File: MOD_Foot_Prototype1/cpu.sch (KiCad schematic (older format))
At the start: 18 parts, among them CN1 CONN_PANNEL_2X2, CN2 CONN_PANNEL_2X2, P1 HEADER_5X2, P2 HEADER_5X2, U2 LPC111X_LQFP48, X1 10MHz

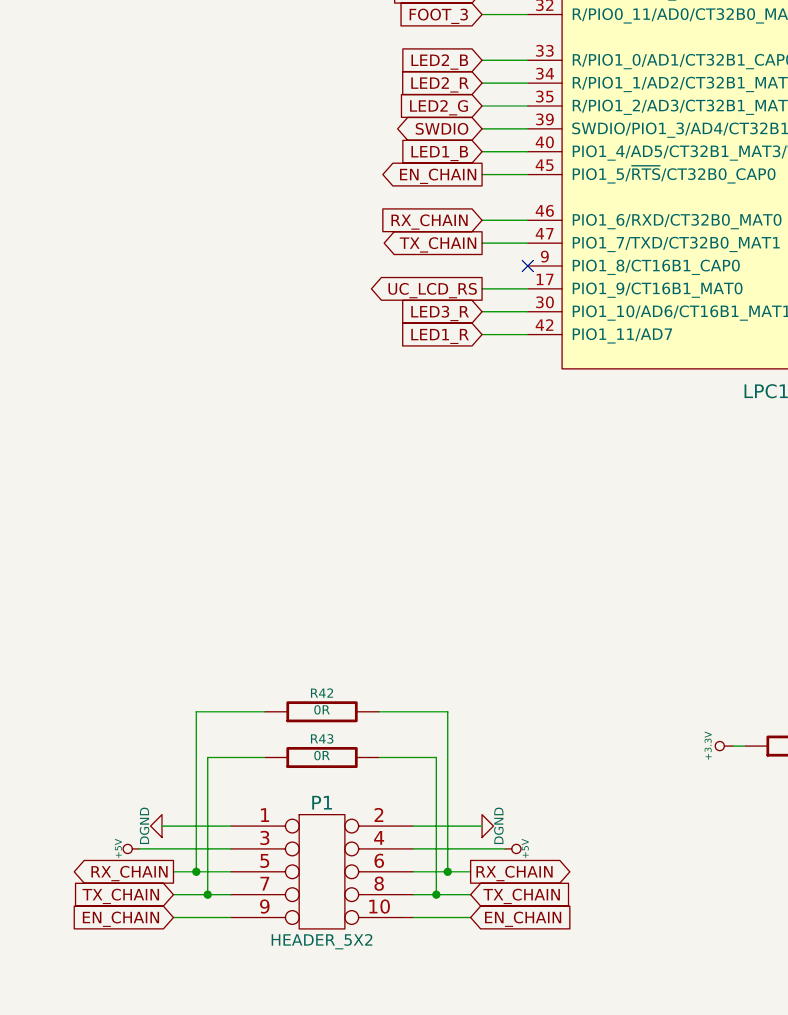
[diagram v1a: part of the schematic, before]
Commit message: yet about issue #11: sch: pins 9 and 10 are being connected with 0R resitor
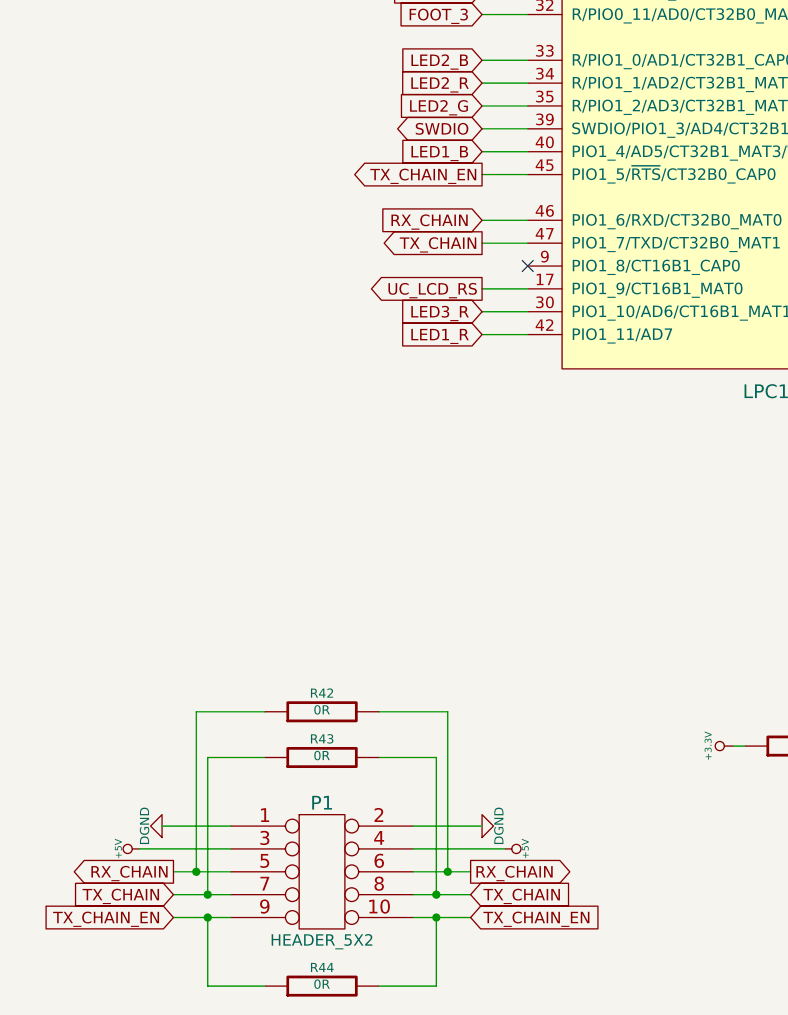
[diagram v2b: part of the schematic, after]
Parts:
- added R44: 0R, MOD_Footprints_Lib:SM0805, symbol R
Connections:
- net EN_CHAIN renamed TX_CHAIN_EN
- net TX_CHAIN_EN: now also R44.1, R44.2
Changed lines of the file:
@@
 RX_CHAIN
 Text GLabel 2650 3450 0    50   Output ~ 0
-EN_CHAIN
+TX_CHAIN_EN
 Text GLabel 2650 3950 0    50   Output ~ 0
 UC_LCD_RS
@@
 $EndComp
 Text GLabel 1300 6700 0    50   Input ~ 0
-EN_CHAIN
+TX_CHAIN_EN
 NoConn ~ 2850 2150
 NoConn ~ 2850 1750
@@
 TX_CHAIN
 Text GLabel 2600 6700 2    50   Input ~ 0
-EN_CHAIN
+TX_CHAIN_EN
 $Comp
 L R R42
@@
 	2500 5800 2500 6500
 Connection ~ 2500 6500
+$Comp
+L R R44
+U 1 1 548854D0
+P 1950 7000
+F 0 "R44" V 2030 7000 40  0000 C CNN
+F 1 "0R" V 1957 7001 40  0000 C CNN
+F 2 "MOD_Footprints_Lib:SM0805" V 1880 7000 30  0001 C CNN
+F 3 "~" H 1950 7000 30  0000 C CNN
+	1    1950 7000
+	0    -1   -1   0
+$EndComp
+Wire Wire Line
+	1700 7000 1450 7000
+Wire Wire Line
+	1450 7000 1450 6700
+Connection ~ 1450 6700
+Wire Wire Line
+	2200 7000 2450 7000
+Wire Wire Line
+	2450 7000 2450 6700
+Connection ~ 2450 6700
 $EndSCHEMATC

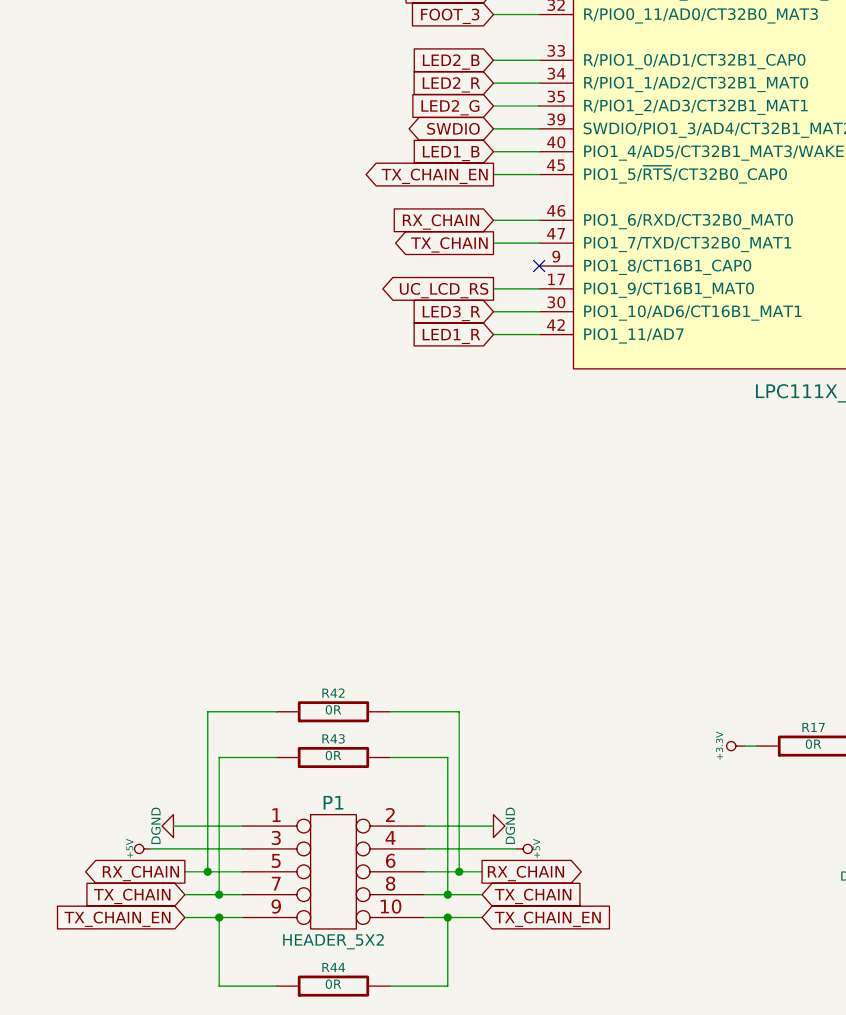
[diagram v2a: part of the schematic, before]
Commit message: * fix wrong control-chain signal names * annotate new resistors added to the sch * rearrange sch drawing around header P1
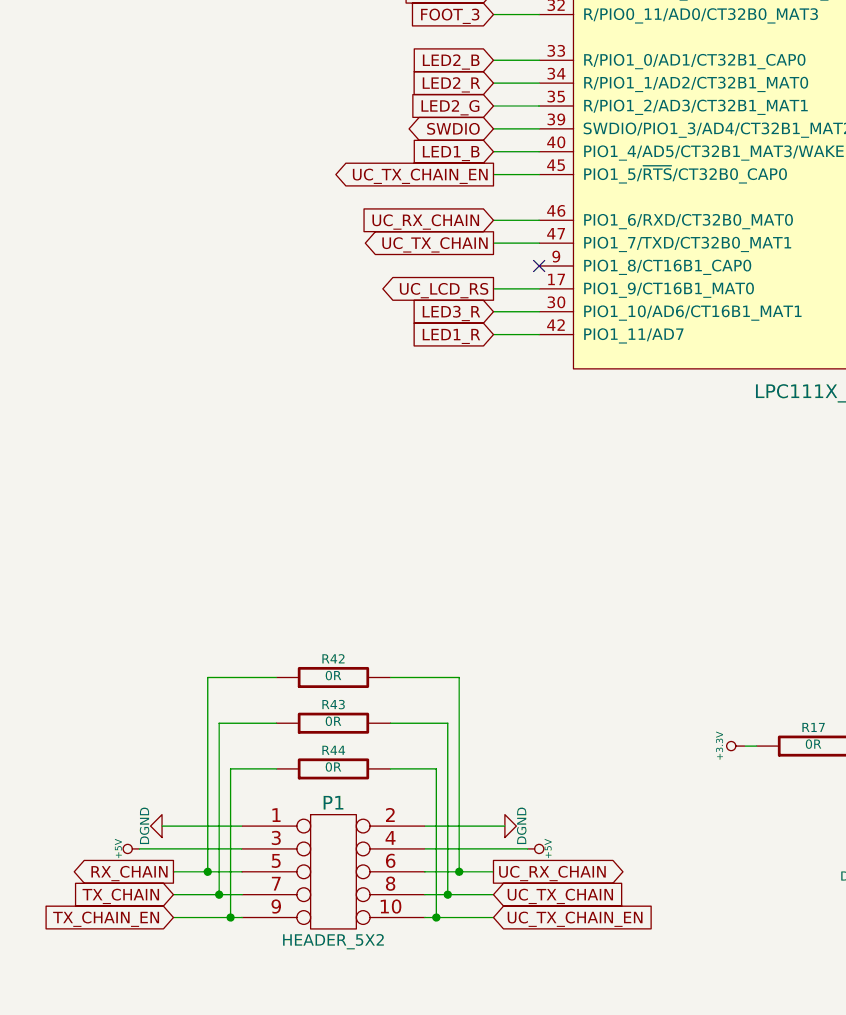
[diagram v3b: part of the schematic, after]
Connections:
- net RX_CHAIN: no longer P1.6, R42.2, U2.46 (PIO1_6/RXD/CT32B0_MAT0)
- net TX_CHAIN: no longer P1.8, R43.2, U2.47 (PIO1_7/TXD/CT32B0_MAT1)
- net TX_CHAIN_EN: no longer P1.10, R44.2, U2.45 (PIO1_5/~RTS~/CT32B0_CAP0)
- new net UC_RX_CHAIN: P1.6, R42.2, U2.46 (PIO1_6/RXD/CT32B0_MAT0)
- new net UC_TX_CHAIN: P1.8, R43.2, U2.47 (PIO1_7/TXD/CT32B0_MAT1)
- new net UC_TX_CHAIN_EN: P1.10, R44.2, U2.45 (PIO1_5/~RTS~/CT32B0_CAP0)
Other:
- moved on the sheet: R42, R43, R44
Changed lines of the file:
@@
 $EndComp
 $Comp
-L DGND #PWR021
+L DGND #PWR30
 U 1 1 54834712
 P 5550 4000
-F 0 "#PWR021" H 5550 4000 40  0001 C CNN
+F 0 "#PWR30" H 5550 4000 40  0001 C CNN
 F 1 "DGND" H 5550 3930 40  0000 C CNN
 F 2 "" H 5550 4000 60  0000 C CNN
@@
 $EndComp
 $Comp
-L DGND #PWR022
+L DGND #PWR35
 U 1 1 5483471F
 P 6550 3600
-F 0 "#PWR022" H 6550 3600 40  0001 C CNN
+F 0 "#PWR35" H 6550 3600 40  0001 C CNN
 F 1 "DGND" H 6550 3530 40  0000 C CNN
 F 2 "" H 6550 3600 60  0000 C CNN
@@
 $EndComp
 $Comp
-L DGND #PWR023
+L DGND #PWR34
 U 1 1 54834725
 P 6550 3400
-F 0 "#PWR023" H 6550 3400 40  0001 C CNN
+F 0 "#PWR34" H 6550 3400 40  0001 C CNN
 F 1 "DGND" H 6550 3330 40  0000 C CNN
 F 2 "" H 6550 3400 60  0000 C CNN
@@
 $EndComp
 $Comp
-L +3.3V #PWR024
+L +3.3V #PWR31
 U 1 1 5483472B
 P 5950 3350
-F 0 "#PWR024" H 5950 3310 30  0001 C CNN
+F 0 "#PWR31" H 5950 3310 30  0001 C CNN
 F 1 "+3.3V" H 5950 3460 30  0000 C CNN
 F 2 "" H 5950 3350 60  0000 C CNN
@@
 $EndComp
 $Comp
-L DGND #PWR025
+L DGND #PWR33
 U 1 1 5483473F
 P 6350 4900
-F 0 "#PWR025" H 6350 4900 40  0001 C CNN
+F 0 "#PWR33" H 6350 4900 40  0001 C CNN
 F 1 "DGND" H 6350 4830 40  0000 C CNN
 F 2 "" H 6350 4900 60  0000 C CNN
@@
 $EndComp
 $Comp
-L DGND #PWR026
+L DGND #PWR32
 U 1 1 54834745
 P 6350 4100
-F 0 "#PWR026" H 6350 4100 40  0001 C CNN
+F 0 "#PWR32" H 6350 4100 40  0001 C CNN
 F 1 "DGND" H 6350 4030 40  0000 C CNN
 F 2 "" H 6350 4100 60  0000 C CNN
@@
 $EndComp
 $Comp
-L DGND #PWR027
+L DGND #PWR24
 U 1 1 54834760
 P 2150 1400
-F 0 "#PWR027" H 2150 1400 40  0001 C CNN
+F 0 "#PWR24" H 2150 1400 40  0001 C CNN
 F 1 "DGND" H 2150 1330 40  0000 C CNN
 F 2 "" H 2150 1400 60  0000 C CNN
@@
 $EndComp
 $Comp
-L +3.3V #PWR028
+L +3.3V #PWR26
 U 1 1 54834766
 P 2750 800
-F 0 "#PWR028" H 2750 760 30  0001 C CNN
+F 0 "#PWR26" H 2750 760 30  0001 C CNN
 F 1 "+3.3V" H 2750 910 30  0000 C CNN
 F 2 "" H 2750 800 60  0000 C CNN
@@
 SWDCLK
 $Comp
-L DGND #PWR029
+L DGND #PWR29
 U 1 1 54834777
 P 4250 6450
-F 0 "#PWR029" H 4250 6450 40  0001 C CNN
+F 0 "#PWR29" H 4250 6450 40  0001 C CNN
 F 1 "DGND" H 4250 6380 40  0000 C CNN
 F 2 "" H 4250 6450 60  0000 C CNN
@@
 NoConn ~ 5150 6250
 Text GLabel 2650 3750 0    50   Output ~ 0
-TX_CHAIN
+UC_TX_CHAIN
 Text GLabel 2650 3650 0    50   Input ~ 0
-RX_CHAIN
+UC_RX_CHAIN
 Text GLabel 2650 3450 0    50   Output ~ 0
-TX_CHAIN_EN
+UC_TX_CHAIN_EN
 Text GLabel 2650 3950 0    50   Output ~ 0
 UC_LCD_RS
@@
 Text GLabel 5650 3100 2    50   Output ~ 0
 LED5
-Text GLabel 1300 6500 0    50   Output ~ 0
+Text GLabel 1250 6500 0    50   Output ~ 0
 RX_CHAIN
-Text GLabel 1300 6600 0    50   Input ~ 0
+Text GLabel 1250 6600 0    50   Input ~ 0
 TX_CHAIN
 $Comp
-L +5V #PWR030
+L +5V #PWR21
 U 1 1 5483479B
-P 1150 6400
-F 0 "#PWR030" H 1150 6490 20  0001 C CNN
-F 1 "+5V" H 1150 6490 30  0000 C CNN
-F 2 "" H 1150 6400 60  0000 C CNN
-F 3 "" H 1150 6400 60  0000 C CNN
-	1    1150 6400
-	0    -1   -1   0
-$EndComp
-$Comp
-L DGND #PWR031
+P 1100 6400
+F 0 "#PWR21" H 1100 6490 20  0001 C CNN
+F 1 "+5V" H 1100 6490 30  0000 C CNN
+F 2 "" H 1100 6400 60  0000 C CNN
+F 3 "" H 1100 6400 60  0000 C CNN
+	1    1100 6400
+	0    -1   -1   0
+$EndComp
+$Comp
+L DGND #PWR22
 U 1 1 548347A1
-P 1250 6300
-F 0 "#PWR031" H 1250 6300 40  0001 C CNN
-F 1 "DGND" H 1250 6225 40  0000 C CNN
-F 2 "" H 1250 6300 60  0000 C CNN
-F 3 "" H 1250 6300 60  0000 C CNN
-	1    1250 6300
+P 1200 6300
+F 0 "#PWR22" H 1200 6300 40  0001 C CNN
+F 1 "DGND" H 1200 6225 40  0000 C CNN
+F 2 "" H 1200 6300 60  0000 C CNN
+F 3 "" H 1200 6300 60  0000 C CNN
+	1    1200 6300
 	0    1    -1   0
 $EndComp
@@
 $EndComp
 $Comp
-L +3.3V #PWR032
+L +3.3V #PWR23
 U 1 1 548347AE
 P 1800 1650
-F 0 "#PWR032" H 1800 1610 30  0001 C CNN
+F 0 "#PWR23" H 1800 1610 30  0001 C CNN
 F 1 "+3.3V" H 1800 1760 30  0000 C CNN
 F 2 "" H 1800 1650 60  0000 C CNN
@@
 $EndComp
 $Comp
-L +3.3V #PWR033
+L +3.3V #PWR28
 U 1 1 54834827
 P 3750 5950
-F 0 "#PWR033" H 3750 5910 30  0001 C CNN
+F 0 "#PWR28" H 3750 5910 30  0001 C CNN
 F 1 "+3.3V" H 3750 6060 30  0000 C CNN
 F 2 "" H 3750 5950 60  0000 C CNN
@@
 	0    -1   -1   0
 $EndComp
-Text GLabel 1300 6700 0    50   Input ~ 0
+Text GLabel 1250 6700 0    50   Input ~ 0
 TX_CHAIN_EN
 NoConn ~ 2850 2150
@@
 NoConn ~ 5450 3300
 $Comp
-L DGND #PWR034
+L DGND #PWR36
 U 1 1 5483484A
 P 7350 5950
-F 0 "#PWR034" H 7350 5950 40  0001 C CNN
+F 0 "#PWR36" H 7350 5950 40  0001 C CNN
 F 1 "DGND" H 7350 5880 40  0000 C CNN
 F 2 "" H 7350 5950 60  0000 C CNN
@@
 $EndComp
 $Comp
-L DGND #PWR035
+L DGND #PWR37
 U 1 1 54834850
 P 8350 5950
-F 0 "#PWR035" H 8350 5950 40  0001 C CNN
+F 0 "#PWR37" H 8350 5950 40  0001 C CNN
 F 1 "DGND" H 8350 5880 40  0000 C CNN
 F 2 "" H 8350 5950 60  0000 C CNN
@@
 $EndComp
 $Comp
-L +5V #PWR036
+L +5V #PWR27
 U 1 1 548788DF
-P 2750 6400
-F 0 "#PWR036" H 2750 6490 20  0001 C CNN
-F 1 "+5V" H 2750 6490 30  0000 C CNN
-F 2 "" H 2750 6400 60  0000 C CNN
-F 3 "" H 2750 6400 60  0000 C CNN
-	1    2750 6400
+P 2800 6400
+F 0 "#PWR27" H 2800 6490 20  0001 C CNN
+F 1 "+5V" H 2800 6490 30  0000 C CNN
+F 2 "" H 2800 6400 60  0000 C CNN
+F 3 "" H 2800 6400 60  0000 C CNN
+	1    2800 6400
 	0    1    -1   0
 $EndComp
 $Comp
-L DGND #PWR037
+L DGND #PWR25
 U 1 1 548788E5
-P 2650 6300
-F 0 "#PWR037" H 2650 6300 40  0001 C CNN
-F 1 "DGND" H 2650 6225 40  0000 C CNN
-F 2 "" H 2650 6300 60  0000 C CNN
-F 3 "" H 2650 6300 60  0000 C CNN
-	1    2650 6300
-	0    -1   -1   0
-$EndComp
-Text GLabel 2600 6500 2    50   Output ~ 0
-RX_CHAIN
-Text GLabel 2600 6600 2    50   Input ~ 0
-TX_CHAIN
-Text GLabel 2600 6700 2    50   Input ~ 0
-TX_CHAIN_EN
+P 2700 6300
+F 0 "#PWR25" H 2700 6300 40  0001 C CNN
+F 1 "DGND" H 2700 6225 40  0000 C CNN
+F 2 "" H 2700 6300 60  0000 C CNN
+F 3 "" H 2700 6300 60  0000 C CNN
+	1    2700 6300
+	0    -1   -1   0
+$EndComp
+Text GLabel 2650 6500 2    50   Output ~ 0
+UC_RX_CHAIN
+Text GLabel 2650 6600 2    50   Input ~ 0
+UC_TX_CHAIN
+Text GLabel 2650 6700 2    50   Input ~ 0
+UC_TX_CHAIN_EN
 $Comp
 L R R42
 U 1 1 54879220
-P 1950 5800
-F 0 "R42" V 2030 5800 40  0000 C CNN
-F 1 "0R" V 1957 5801 40  0000 C CNN
-F 2 "MOD_Footprints_Lib:SM0805" V 1880 5800 30  0001 C CNN
-F 3 "~" H 1950 5800 30  0000 C CNN
-	1    1950 5800
+P 1950 5650
+F 0 "R42" V 2030 5650 40  0000 C CNN
+F 1 "0R" V 1957 5651 40  0000 C CNN
+F 2 "MOD_Footprints_Lib:SM0805" V 1880 5650 30  0001 C CNN
+F 3 "~" H 1950 5650 30  0000 C CNN
+	1    1950 5650
 	0    -1   -1   0
 $EndComp
@@
 L R R43
 U 1 1 548792F8
-P 1950 6000
-F 0 "R43" V 2030 6000 40  0000 C CNN
-F 1 "0R" V 1957 6001 40  0000 C CNN
-F 2 "MOD_Footprints_Lib:SM0805" V 1880 6000 30  0001 C CNN
-F 3 "~" H 1950 6000 30  0000 C CNN
-	1    1950 6000
+P 1950 5850
+F 0 "R43" V 2030 5850 40  0000 C CNN
+F 1 "0R" V 1957 5851 40  0000 C CNN
+F 2 "MOD_Footprints_Lib:SM0805" V 1880 5850 30  0001 C CNN
+F 3 "~" H 1950 5850 30  0000 C CNN
+	1    1950 5850
 	0    -1   -1   0
 $EndComp
@@
 	2650 3450 2850 3450
 Wire Wire Line
-	1150 6400 1550 6400
-Wire Wire Line
-	1250 6300 1550 6300
+	1100 6400 1550 6400
+Wire Wire Line
+	1200 6300 1550 6300
 Wire Wire Line
 	1800 1650 1850 1650
@@
 Connection ~ 7350 5400
 Wire Wire Line
-	1300 6500 1550 6500
-Wire Wire Line
-	1300 6600 1550 6600
-Wire Wire Line
-	1300 6700 1550 6700
-Wire Wire Line
-	2750 6400 2350 6400
-Wire Wire Line
-	2650 6300 2350 6300
-Wire Wire Line
-	2350 6500 2600 6500
-Wire Wire Line
-	2600 6600 2350 6600
-Wire Wire Line
-	2350 6700 2600 6700
-Wire Wire Line
-	1700 6000 1450 6000
-Wire Wire Line
-	1450 6000 1450 6600
+	1250 6500 1550 6500
+Wire Wire Line
+	1250 6600 1550 6600
+Wire Wire Line
+	1250 6700 1550 6700
+Wire Wire Line
+	2350 6400 2800 6400
+Wire Wire Line
+	2350 6300 2700 6300
+Wire Wire Line
+	2350 6500 2650 6500
+Wire Wire Line
+	2350 6600 2650 6600
+Wire Wire Line
+	2350 6700 2650 6700
+Wire Wire Line
+	1700 5850 1450 5850
+Wire Wire Line
+	1450 5850 1450 6600
 Connection ~ 1450 6600
 Wire Wire Line
-	1700 5800 1400 5800
-Wire Wire Line
-	1400 5800 1400 6500
+	1700 5650 1400 5650
+Wire Wire Line
+	1400 5650 1400 6500
 Connection ~ 1400 6500
 Wire Wire Line
-	2200 6000 2450 6000
-Wire Wire Line
-	2450 6000 2450 6600
+	2200 5850 2450 5850
+Wire Wire Line
+	2450 5850 2450 6600
 Connection ~ 2450 6600
 Wire Wire Line
-	2200 5800 2500 5800
-Wire Wire Line
-	2500 5800 2500 6500
+	2200 5650 2500 5650
+Wire Wire Line
+	2500 5650 2500 6500
 Connection ~ 2500 6500
 $Comp
 L R R44
 U 1 1 548854D0
-P 1950 7000
-F 0 "R44" V 2030 7000 40  0000 C CNN
-F 1 "0R" V 1957 7001 40  0000 C CNN
-F 2 "MOD_Footprints_Lib:SM0805" V 1880 7000 30  0001 C CNN
-F 3 "~" H 1950 7000 30  0000 C CNN
-	1    1950 7000
-	0    -1   -1   0
-$EndComp
-Wire Wire Line
-	1700 7000 1450 7000
-Wire Wire Line
-	1450 7000 1450 6700
-Connection ~ 1450 6700
-Wire Wire Line
-	2200 7000 2450 7000
-Wire Wire Line
-	2450 7000 2450 6700
-Connection ~ 2450 6700
+P 1950 6050
+F 0 "R44" V 2030 6050 40  0000 C CNN
+F 1 "0R" V 1957 6051 40  0000 C CNN
+F 2 "MOD_Footprints_Lib:SM0805" V 1880 6050 30  0001 C CNN
+F 3 "~" H 1950 6050 30  0000 C CNN
+	1    1950 6050
+	0    -1   -1   0
+$EndComp
+Wire Wire Line
+	1500 6700 1500 6050
+Wire Wire Line
+	1500 6050 1700 6050
+Connection ~ 1500 6700
+Wire Wire Line
+	2400 6700 2400 6050
+Wire Wire Line
+	2400 6050 2200 6050
+Connection ~ 2400 6700
 $EndSCHEMATC
